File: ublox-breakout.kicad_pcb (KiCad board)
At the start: 4 copper layers, 30 parts, among them J1 Conn_Coaxial, J2 Conn_01x07, J3 Conn_01x07, U1 AT2659S, U2 SAFFB1G56KB0F0A, U3 UBX-G7020-KT, X1 26MHz, Y1 32.768k

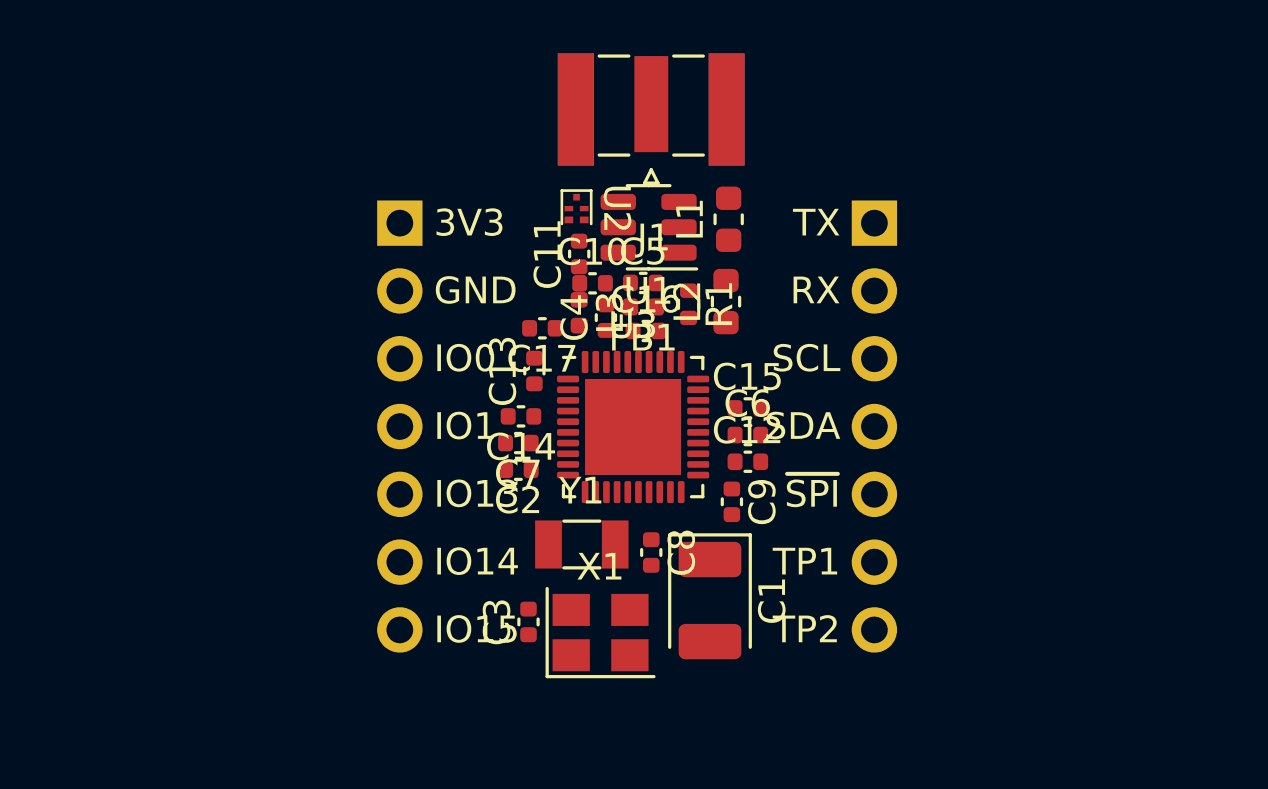
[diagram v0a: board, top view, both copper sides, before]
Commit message: Finish layout
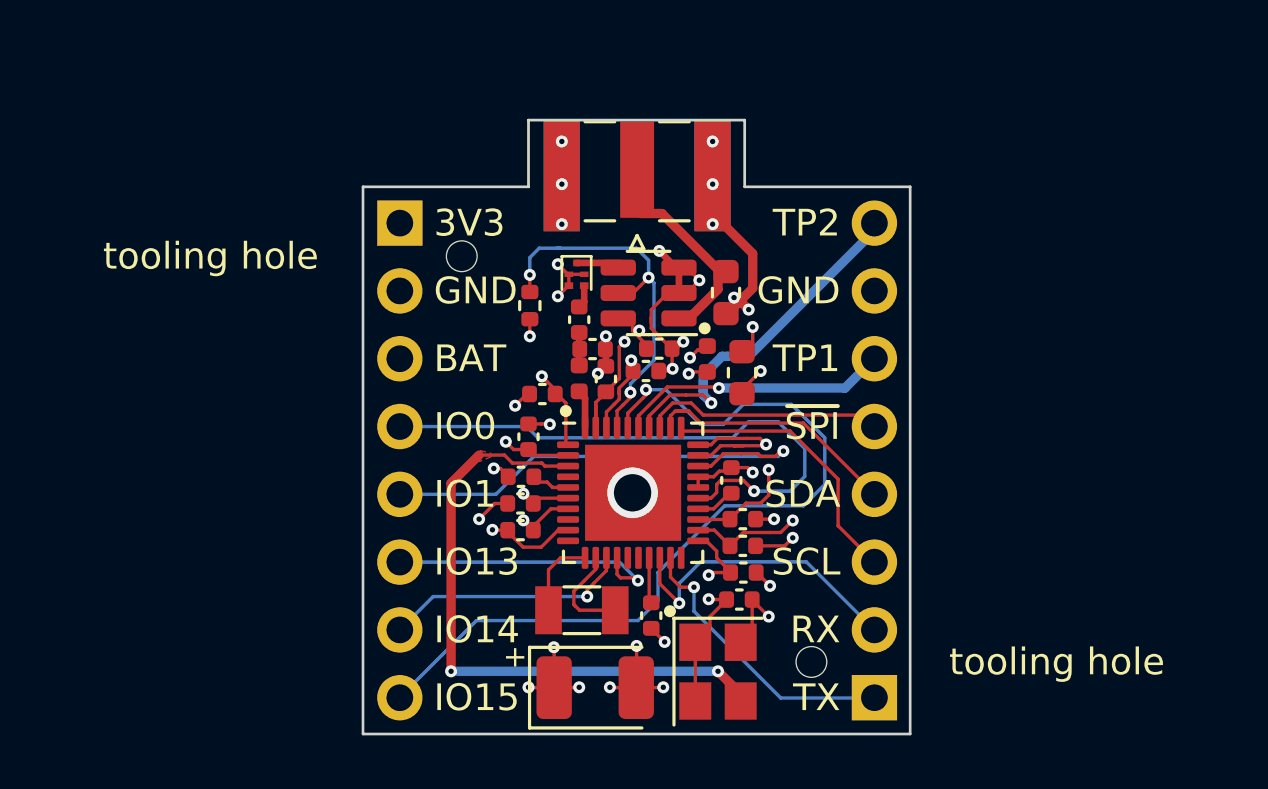
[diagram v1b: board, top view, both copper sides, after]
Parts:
- added H1: ToolingHole, ToolingHole:ToolingHole_JLCSMT, F.Cu at (96.3, 87.6)
- added H2: ToolingHole, ToolingHole:ToolingHole_JLCSMT, F.Cu at (109.4, 102.8)
- J2, J3: value Conn_01x07 -> Conn_01x08; footprint Connector_PinHeader_2.54mm:PinHeader_1x07_P2.54mm_Vertical -> Connector_PinHeader_2.54mm:PinHeader_1x08_P2.54mm_Vertical
- moved J3 25.1 mm to (111.8, 104.1), turned to 0 degrees
- moved J2 17.8 mm to (94.0, 86.4)
- moved C3 7.94 mm to (106.7, 100.5), turned to 0 degrees
- moved R1 5.95 mm to (98.8, 89.5), turned to 90 degrees
- moved C1 5.40 mm to (101.3, 103.8), turned to 0 degrees
- moved X1 4.64 mm to (105.9, 103.2), turned to -90 degrees
- moved C12 3.16 mm to (106.8, 98.5)
- moved C6 3.16 mm to (106.8, 97.5)
- moved FB1 3.09 mm to (105.5, 91.5), turned to 90 degrees
- moved C15 2.77 mm to (106.4, 96.0), turned to 90 degrees
- moved L1 2.75 mm to (106.2, 89.0)
- moved L2 2.73 mm to (106.8, 92.0)
- moved C9 2.68 mm to (106.8, 99.5), turned to 0 degrees
- moved C5 2.53 mm to (103.7, 91.1)
- moved J1 2.52 mm to (102.9, 84.6)
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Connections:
- J2 pad 1: /TX -> +3V3
- J2 pad 2: /RX -> GND
- J2 pad 3: /SCL -> +BATT
- J2 pad 4: /SDA -> /PIO0
- J2 pad 5: /~{SPI_EN} -> /PIO1
- J2 pad 6: /TIME1 -> /PIO13
- J2 pad 7: /TIME2 -> /PIO14
- J3 pad 1: +3V3 -> /TX
- J3 pad 2: GND -> /RX
- J3 pad 3: /PIO0 -> /SCL
- J3 pad 4: /PIO1 -> /SDA
- J3 pad 5: /PIO13 -> /~{SPI_EN}
- J3 pad 6: /PIO14 -> /TIME1
- J3 pad 7: /PIO15 -> GND
- U2 pad 2: (no net) -> GND
- U2 pad 3: (no net) -> GND
- U2 pad 5: (no net) -> GND
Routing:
- net GND: track 0.00 -> 46.7 mm, vias 0 -> 33
- net /PIO15: track 0.00 -> 31.4 mm, vias 0 -> 1
- net Net-(U3-Pad3): track 0.00 -> 24.1 mm, vias 0 -> 2
- net /PIO0: track 0.00 -> 22.5 mm, vias 0 -> 1
- net +1V8: track 0.00 -> 18.8 mm, vias 0 -> 2
- net /PIO1: track 0.00 -> 18.5 mm, vias 0 -> 1
- net +3V3: track 0.00 -> 17.5 mm, vias 0 -> 8
- net Net-(C4-Pad1): track 0.00 -> 14.8 mm, vias 0 -> 3
- net /LNA_ON: track 0.00 -> 14.5 mm, vias 0 -> 3
- net /TIME2: track 0.00 -> 14.1 mm, vias 0 -> 1
- net /RX: track 0.00 -> 11.4 mm, vias 0 -> 1
- net /TX: track 0.00 -> 10.8 mm, vias 0 -> 1
- net /PIO13: track 0.00 -> 10.7 mm, vias 0 -> 1
- net /SCL: track 0.00 -> 10.3 mm
- net /TIME1: track 0.00 -> 10.3 mm, vias 0 -> 1
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- added copper zone on In2.Cu, net +3V3
- added copper zone on In1.Cu, net GND
- added copper zone on F.Cu, net Net-(U3-Pad3)
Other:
- board outline added: 20.5 x 23 mm
- board text added: "+"
- board text added: "BAT"
- board text added: "Designed by Tobias Schramm in 2022"
- board text added: "JLCJLCJLCJLC"
- board text added: "u-blox M8030 Breakout Rev 1.0"
